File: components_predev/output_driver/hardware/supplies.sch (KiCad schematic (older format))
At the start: 3 parts

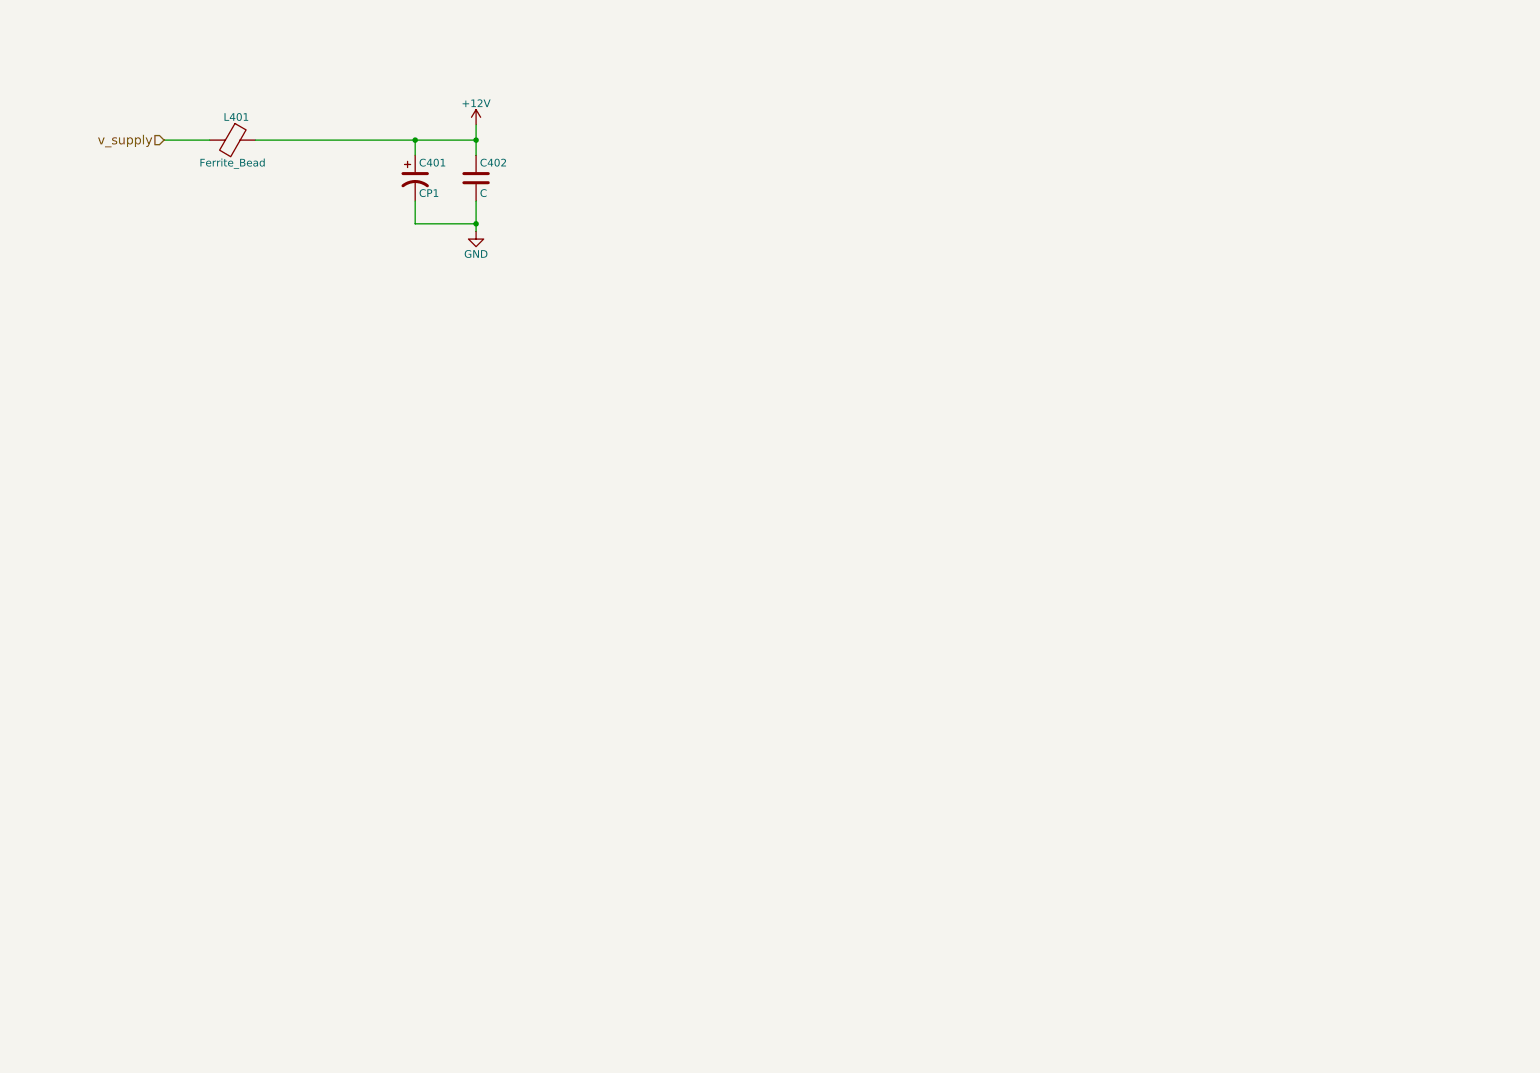
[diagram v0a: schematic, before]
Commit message: Added Supply Schematic
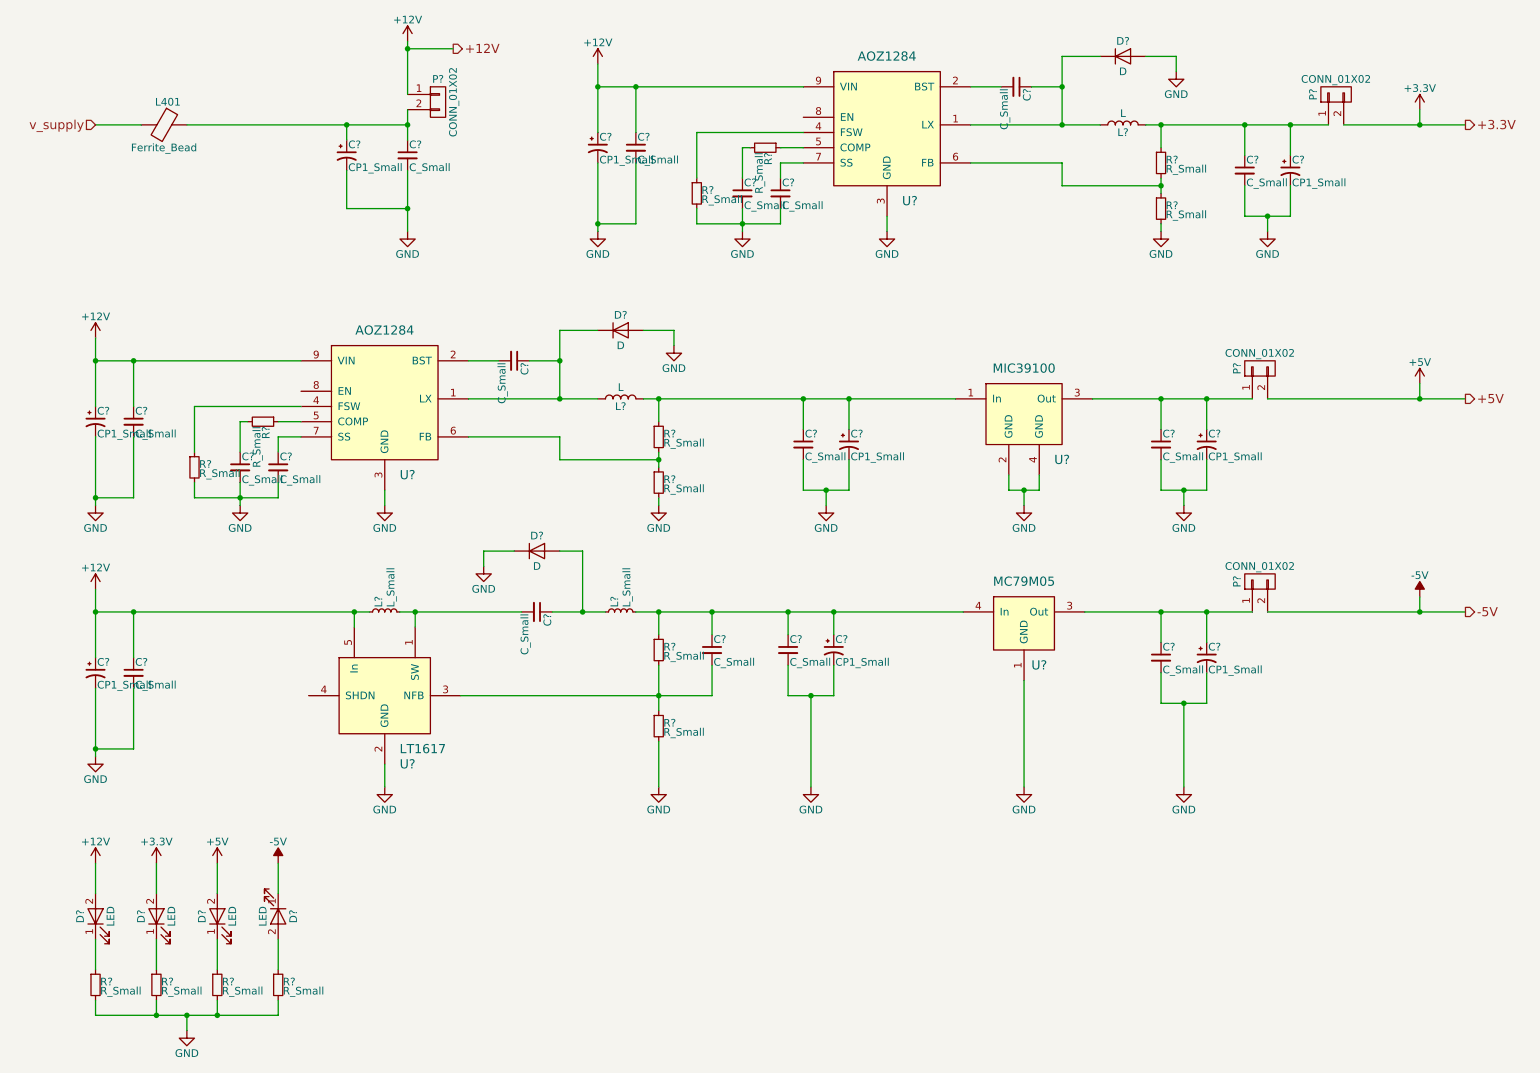
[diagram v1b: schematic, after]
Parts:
- removed C401: CP1, symbol CP1
- removed C402: C, symbol C
- added C? (x17): C_Small, symbol C_Small
- added C? (x9): CP1_Small, symbol CP1_Small
- added D? (x3): D, symbol D
- added D? (x4): LED, symbol LED
- added L? (x2): L, symbol L
- added L? (x2): L_Small, symbol L_Small
- added P? (x4): CONN_01X02, symbol CONN_01X02
- added R? (x14): R_Small, symbol R_Small
- added U? (x2): AOZ1284, symbol AOZ1284
- added U?: MIC39100, symbol MIC39100
- added U?: LT1617, symbol LT1617
- added U?: MC79M05, symbol MC79M05
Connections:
- net +12V: now also C?.1, C?.1, C?.1, C?.1, C?.1, C?.1, D?.2 (A), L?.1, P?.1 (P1), U?.5 (In), U?.9 (VIN), U?.9 (VIN); no longer L401.1
- net GND: now also C?.2, C?.2, C?.2, C?.2, C?.2, C?.2, C?.2, C?.2, C?.2, C?.2, C?.2, C?.2, C?.2, C?.2, C?.2, C?.2, C?.2, C?.2, C?.2, C?.2, C?.2, C?.2, D?.1 (K), D?.2 (A), D?.2 (A), R?.2, R?.2, R?.2, R?.2, R?.2, R?.2, R?.2, R?.2, R?.2, U?.1 (GND), U?.2 (GND), U?.2 (GND), U?.3 (GND), U?.3 (GND), U?.4 (GND)
- new net: C?.1, C?.1, L401.1, P?.2 (P2)
- new net: C?.1, D?.1 (K), L?.1, U?.1 (LX) (x2)
- new net: C?.2, U?.2 (BST) (x2)
- new net: R?.1, U?.4 (FSW) (x2)
- new net: R?.1, U?.5 (COMP) (x2)
- new net: R?.1, R?.2, U?.6 (FB) (x2)
- new net: C?.1, U?.7 (SS) (x2)
- new net: C?.1, C?.1, L?.2, P?.1 (P1), R?.1
- new net: C?.1, R?.2 (x2)
- new net: C?.1, C?.1, L?.2, R?.1, U?.1 (In)
- new net: C?.1, C?.1, P?.1 (P1), U?.3 (Out) (x2)
- new net: D?.1 (K), R?.1 (x3)
- new net: D?.2 (A), R?.1
- new net: C?.2, L?.2, U?.1 (SW)
- new net: C?.2, R?.1, R?.2, U?.3 (NFB)
- new net: C?.1, D?.2 (A), L?.1
- new net: C?.1, C?.1, C?.1, L?.2, R?.1, U?.4 (In)
- new net +3V3: D?.2 (A), P?.2 (P2)
- new net +5V: D?.2 (A), P?.2 (P2)
- new net -5V: D?.1 (K), P?.2 (P2)
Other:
- moved on the sheet: L401
